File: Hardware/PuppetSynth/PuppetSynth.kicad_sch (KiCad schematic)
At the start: 22 parts, among them J1 ADS1115, J2 ADS1115, SW1 SW_Rotary_1x4_MP, SW2 SW_Rotary_1x4_MP, SW3 SW_Rotary_1x4_MP, SW4 SW_SP3T_NR01103, SW5 SW_SP3T_NR01103, SW6 SW_SP3T_NR01103, SW7 Switch

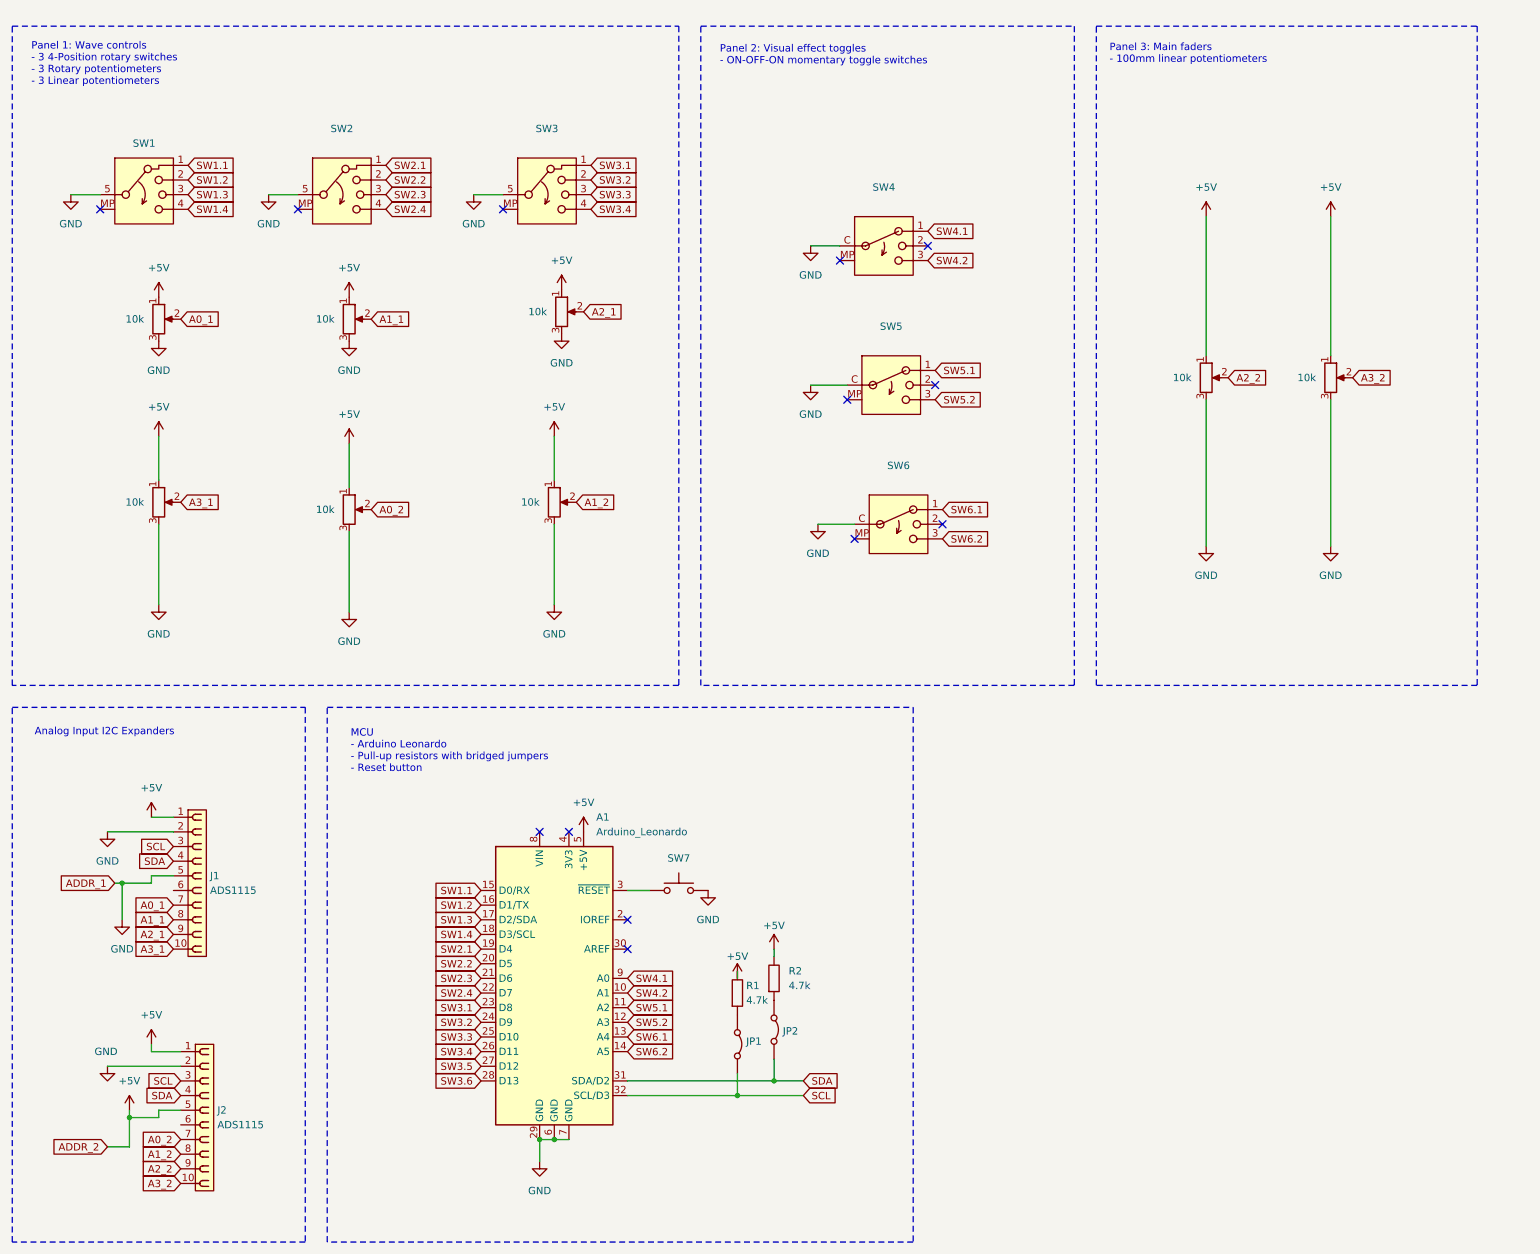
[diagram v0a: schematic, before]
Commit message: updated and exported schematic
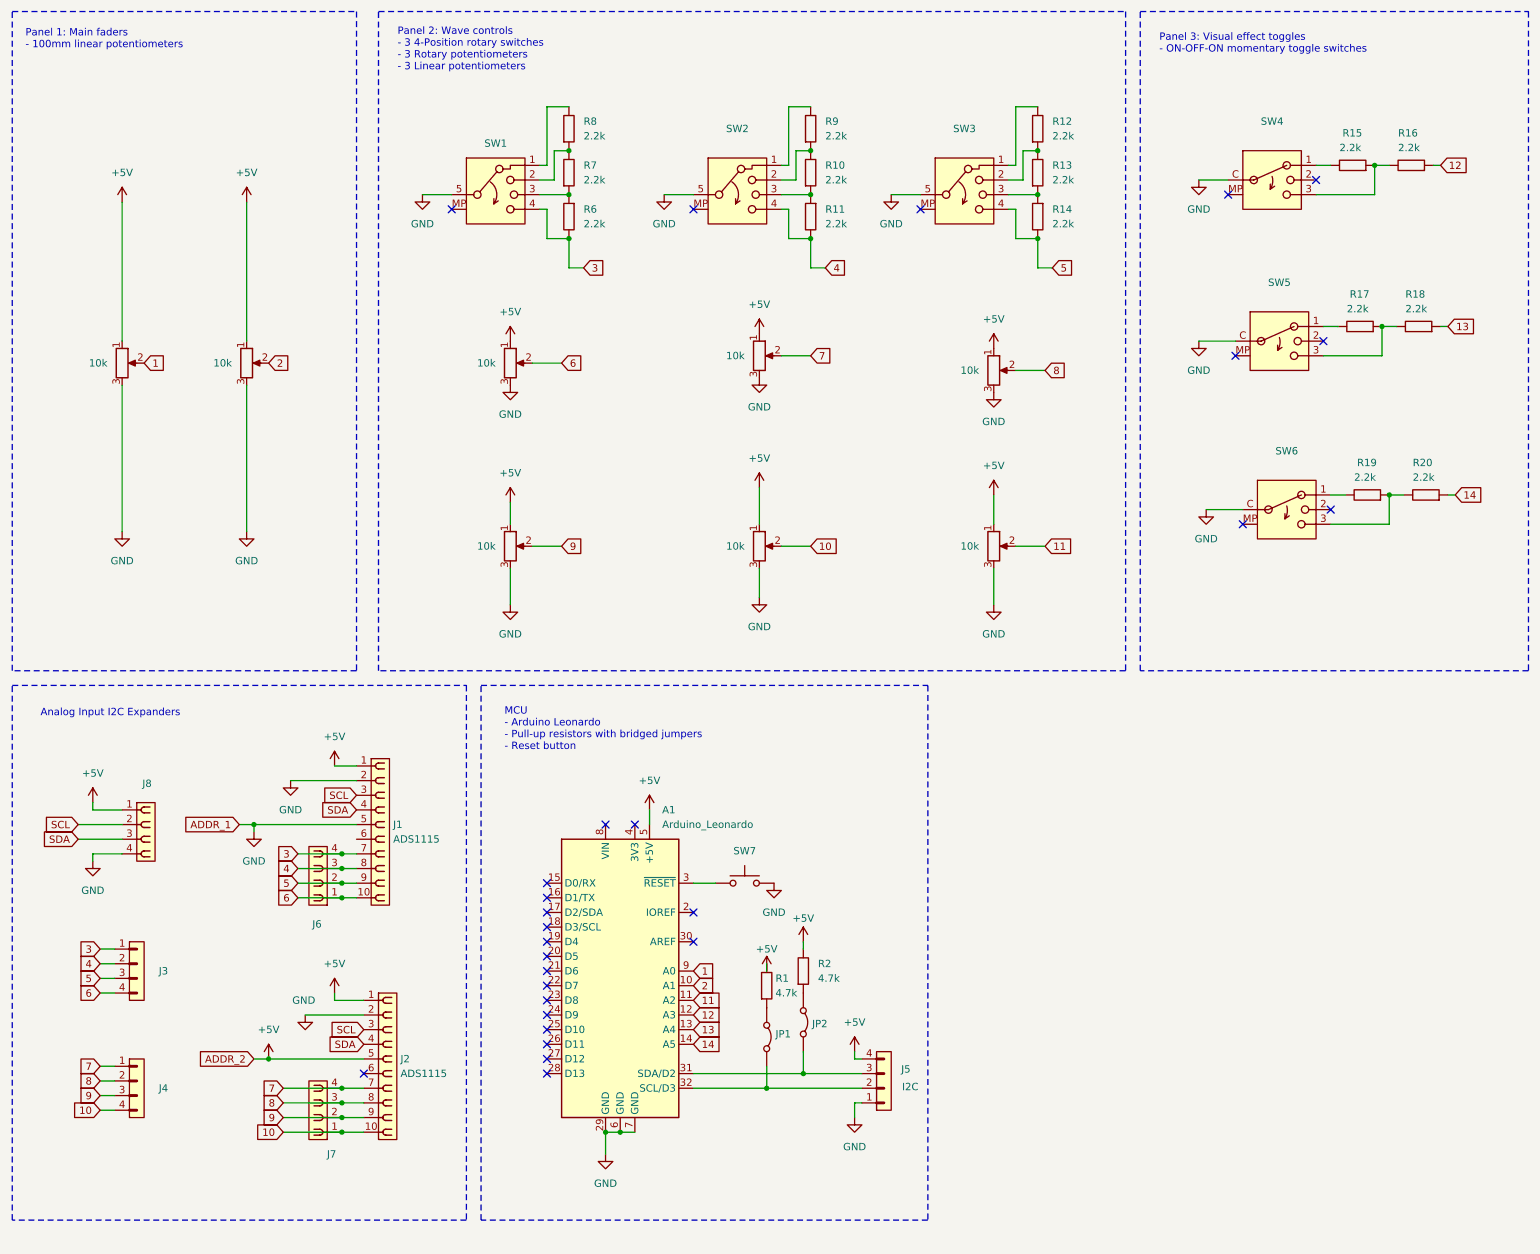
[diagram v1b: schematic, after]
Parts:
- added J3, J4: PINHD_1x4_Male, Connector_PinHeader_2.54mm:PinHeader_1x04_P2.54mm_Vertical, symbol PCM_SL_Pin_Headers:PINHD_1x4_Male
- added J5: I2C, Connector_PinHeader_2.54mm:PinHeader_1x04_P2.54mm_Vertical, symbol PCM_SL_Pin_Headers:PINHD_1x4_Male
- added J6, J7, J8: PINHD_1x4_Female, Connector_PinSocket_2.54mm:PinSocket_1x04_P2.54mm_Vertical, symbol PCM_SL_Pin_Headers:PINHD_1x4_Female
- added R10, R11, R12, R13, R14, R15, R16, R17, R18, R19, R20, R6, R7, R8, R9: 2.2k, Resistor_THT:R_Axial_DIN0207_L6.3mm_D2.5mm_P10.16mm_Horizontal, symbol PCM_SL_Resistors:2.2k
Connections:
- net +5V: now also J5.4, J8.1
- net GND: now also J5.1, J8.4
- net SCL: now also J8.2; no longer A1.32 (SCL/D3), JP1.2 (B)
- net SDA: now also J8.3; no longer A1.31 (SDA/D2), JP2.2 (B)
- net A0_1 renamed 3
- net 3: now also SW1.4, J3.1, J6.4, R6.2; no longer 10k.2
- net A0_2 renamed 10
- net 10: now also J2.10, J4.4, J7.1; no longer J2.7
- net A1_1 renamed 4
- net 4: now also SW2.4, J3.2, J6.3, R11.2; no longer 10k.2
- net A1_2 renamed 11
- net 11: now also A1.11 (A2); no longer J2.8
- net A2_1 renamed 5
- net 5: now also SW3.4, J3.3, J6.2, R14.2; no longer 10k.2
- net A2_2 renamed 1
- net 1: now also A1.9 (A0); no longer J2.9
- net A3_1 renamed 6
- net 6: now also 10k.2, J3.4, J6.1; no longer 10k.2
- net A3_2 renamed 2
- net 2: now also A1.10 (A1); no longer J2.10
- net SW1.1: no longer names the net of A1.15 (D0/RX)
- net SW1.1: no longer SW1.1
- net SW1.2: no longer names the net of A1.16 (D1/TX)
- net SW1.2: no longer SW1.2
- net SW1.3: no longer names the net of A1.17 (D2/SDA)
- net SW1.3: no longer SW1.3
- net SW1.4: no longer names the net of A1.18 (D3/SCL)
- net SW1.4: no longer SW1.4
- net SW2.1: no longer names the net of SW2.1
- net SW2.1: now also R9.2; no longer A1.19 (D4)
- net SW2.2: no longer names the net of SW2.2
- net SW2.2: now also R10.2, R9.1; no longer A1.20 (D5)
- net SW2.3: no longer names the net of SW2.3
- net SW2.3: now also R10.1, R11.1; no longer A1.21 (D6)
- net SW2.4: no longer names the net of A1.22 (D7)
- net SW2.4: no longer SW2.4
- net SW3.1: no longer names the net of A1.23 (D8)
- net SW3.1: no longer SW3.1
- net SW3.2: no longer names the net of A1.24 (D9)
- net SW3.2: no longer SW3.2
- net SW3.3: no longer names the net of SW3.3
- net SW3.3: now also R13.1, R14.1; no longer A1.25 (D10)
- net SW3.4: no longer names the net of A1.26 (D11)
- net SW3.4: no longer SW3.4
- net SW3.5: no longer names the net of A1.27 (D12)
- net SW3.6: no longer names the net of A1.28 (D13)
- net SW4.1: no longer names the net of SW4.1
- net SW4.1: now also R15.2; no longer A1.9 (A0)
- net SW4.2: no longer names the net of SW4.3
- net SW4.2: now also R15.1, R16.2; no longer A1.10 (A1)
- net SW5.1: no longer names the net of SW5.1
- net SW5.1: now also R17.2; no longer A1.11 (A2)
- net SW5.2: no longer names the net of SW5.3
- net SW5.2: now also R17.1, R18.2; no longer A1.12 (A3)
- net SW6.1: no longer names the net of SW6.1
- net SW6.1: now also R19.2; no longer A1.13 (A4)
- net SW6.2: no longer names the net of SW6.3
- net SW6.2: now also R19.1, R20.2; no longer A1.14 (A5)
- new net: A1.31 (SDA/D2), J5.3, JP2.2 (B)
- new net: A1.32 (SCL/D3), J5.2, JP1.2 (B)
- new net: R7.2, R8.1, SW1.2
- new net: R8.2, SW1.1
- new net: R12.2, SW3.1
- new net: R12.1, R13.2, SW3.2
- new net: R6.1, R7.1, SW1.3
- new net 12: A1.12 (A3), R16.1
- new net 13: A1.13 (A4), R18.1
- new net 14: A1.14 (A5), R20.1
- new net 7: 10k.2, J2.7, J4.1, J7.4
- new net 8: 10k.2, J2.8, J4.2, J7.3
- new net 9: 10k.2, J2.9, J4.3, J7.2
- no-connect marks 13 -> 28
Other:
- note added: "Panel 1: Main faders - 100mm linear potentiometers"
- note added: "Panel 2: Wave controls - 3 4-Position rotary switches - 3 Rotary potentiometers - 3 Linear potentiometers"
- note added: "Panel 3: Visual effect toggles - ON-OFF-ON momentary toggle switches"
- note removed: "Panel 1: Wave controls - 3 4-Position rotary switches - 3 Rotary potentiometers - 3 Linear potentiometers"
- note removed: "Panel 2: Visual effect toggles - ON-OFF-ON momentary toggle switches"
- note removed: "Panel 3: Main faders - 100mm linear potentiometers"
- moved on the sheet: 10k, A1, J1, J2, JP1, JP2, R1, R2, SW1, SW2, SW3, SW4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
